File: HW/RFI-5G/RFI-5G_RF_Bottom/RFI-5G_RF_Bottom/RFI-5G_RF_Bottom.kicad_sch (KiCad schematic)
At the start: 20 parts, among them J1 Conn_01x10, J2 Conn_01x10, J3 Conn_01x10, J4 Conn_01x10, J5 SMP, J6 Conn_01x04_Female

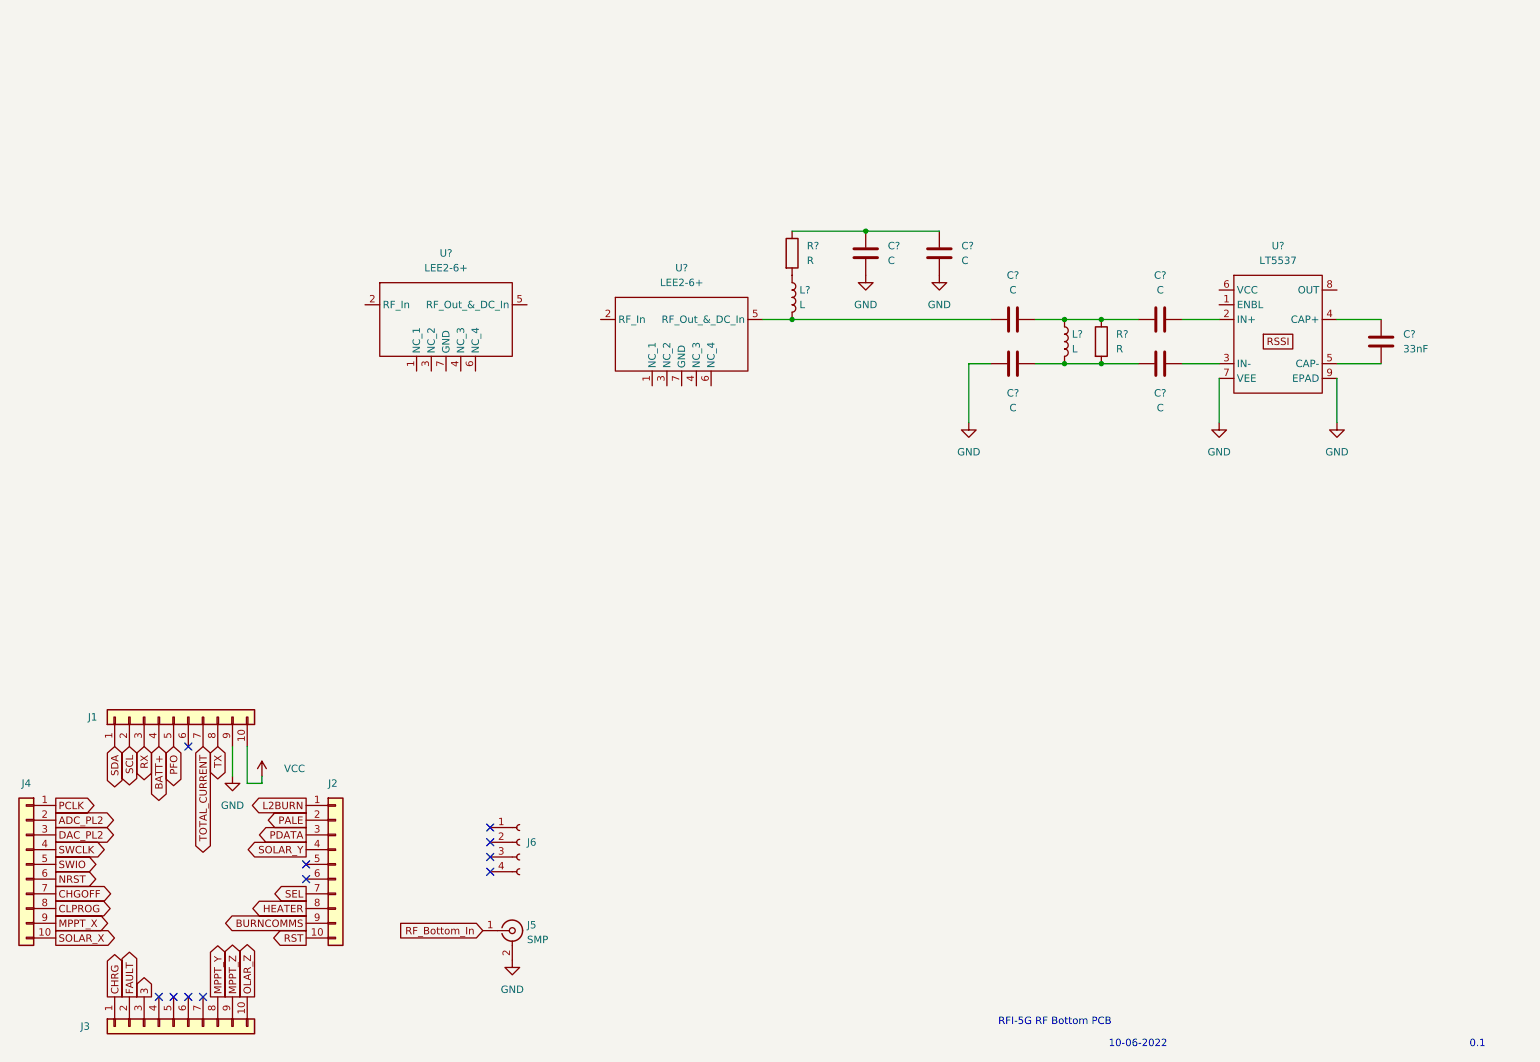
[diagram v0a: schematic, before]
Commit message: RF top and Bottom boards
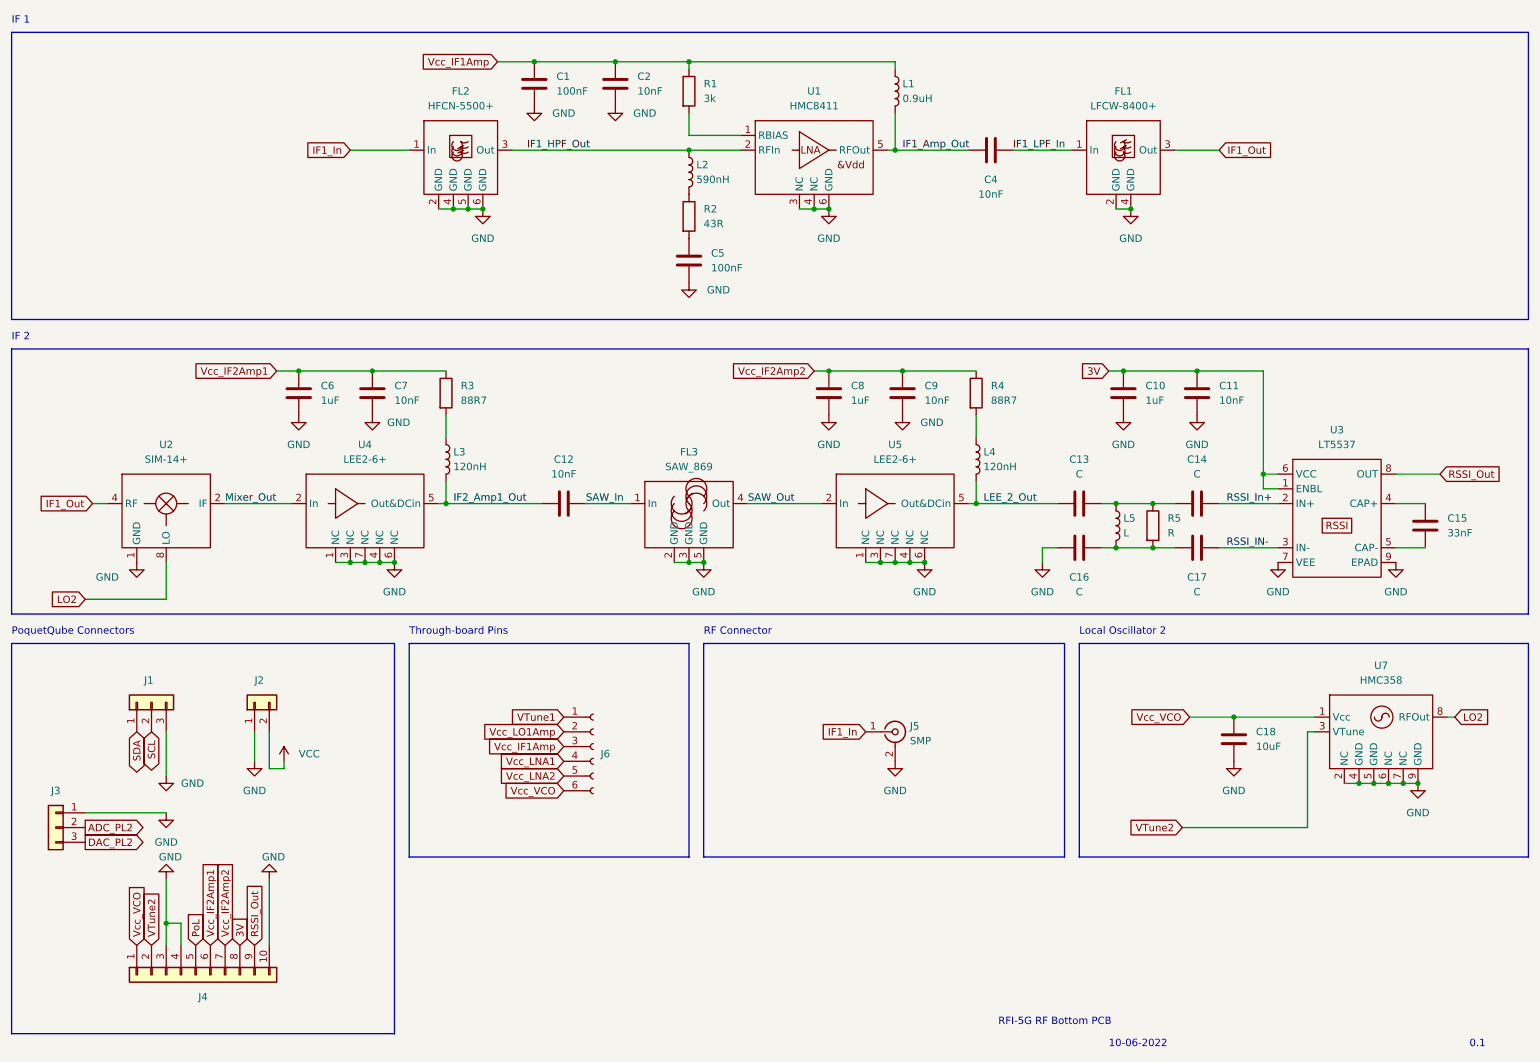
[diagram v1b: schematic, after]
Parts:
- removed J1, J2, J3: Conn_01x10, symbol Connector_Generic:Conn_01x10
- removed J6: Conn_01x04_Female, Connector_PinHeader_2.54mm:PinHeader_1x04_P2.54mm_Vertical, symbol Connector:Conn_01x04_Female
- removed U?: LEE2-6+, Package_SON:WSON-6-1EP_2x2mm_P0.65mm_EP1x1.6mm, symbol GGS_RF:LEE2-6+
- added C1, C5: 100nF, Capacitor_SMD:C_0402_1005Metric, symbol Device:C
- added C10, C6: 1uF, Capacitor_SMD:C_0402_1005Metric, symbol Device:C
- added C11, C12, C2, C4, C7: 10nF, Capacitor_SMD:C_0402_1005Metric, symbol Device:C
- added C18: 10uF, Capacitor_SMD:C_0402_1005Metric, symbol Device:C
- added FL1: LFCW-8400+, GGS_RF:JC0603C-1, symbol GGS_RF:LFCW-8000+
- added FL2: HFCN-5500+, GGS_RF:JC0603C, symbol GGS_RF:HFCN-5500+
- added FL3: SAW_869, GGS_RF:QCS5P, symbol GGS_RF:SAW_869
- added J1, J3: Conn_01x03, Connector_PinHeader_2.54mm:PinHeader_1x03_P2.54mm_Vertical, symbol Connector_Generic:Conn_01x03
- added J2: Conn_01x02, Connector_PinHeader_2.54mm:PinHeader_1x02_P2.54mm_Vertical, symbol Connector_Generic:Conn_01x02
- added J6: Conn_01x06_Female, Connector_PinHeader_1.00mm:PinHeader_1x06_P1.00mm_Vertical, symbol Connector:Conn_01x06_Female
- added L1: 0.9uH, Inductor_SMD:L_0603_1608Metric, symbol Device:L
- added L2: 590nH, Inductor_SMD:L_0603_1608Metric, symbol Device:L
- added L3: 120nH, Inductor_SMD:L_0603_1608Metric, symbol Device:L
- added R1: 3k, Resistor_SMD:R_0603_1608Metric, symbol Device:R
- added R2: 43R, Resistor_SMD:R_0603_1608Metric, symbol Device:R
- added R3: 88R7, Resistor_SMD:R_0603_1608Metric, symbol Device:R
- added U1: HMC8411, GGS_RF:6-LFCSP, symbol GGS_RF:HMC8411
- added U2: SIM-14+, GGS_RF:HV1195, symbol GGS_RF:SIM-14+
- added U4: LEE2-6+, Package_SON:WSON-6-1EP_2x2mm_P0.65mm_EP1x1.6mm, symbol GGS_RF:LEE2-6+
- added U7: HMC358, Package_SO:MSOP-8-1EP_3x3mm_P0.65mm_EP2.5x3mm_Mask1.73x2.36mm, symbol GGS_RF:HMC358
- C8: renamed from C?; value C -> 1uF
- C9: renamed from C?; value C -> 10nF
- J4: footprint (none) -> Connector_PinHeader_2.54mm:PinHeader_1x10_P2.54mm_Vertical
- J5: footprint easyeda:CES-110-XX-Y-S -> GGS_Connectors:SMP_StraightPlugPCB
- L4: renamed from L?; value L -> 120nH; footprint (none) -> Inductor_SMD:L_0603_1608Metric
- L5: renamed from L?; footprint (none) -> Inductor_SMD:L_0603_1608Metric
- R4: renamed from R?; value R -> 88R7; footprint (none) -> Resistor_SMD:R_0603_1608Metric
- R5: renamed from R?; footprint (none) -> Resistor_SMD:R_0603_1608Metric
- gave numbers to parts that had none: 7
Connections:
- net CHGOFF is gone; now on net Vcc_IF2Amp2: J4.7 (Pin_7)
- net CLPROG is gone; now on net 3V: J4.8 (Pin_8)
- net MPPT_X is gone; now on net RSSI_Out: J4.9 (Pin_9)
- net SOLAR_X is gone; now on net GND: J4.10 (Pin_10)
- net SWCLK is gone; now on net GND: J4.4 (Pin_4)
- net ADC_PL2: now also J3.2 (Pin_2); no longer J4.2 (Pin_2)
- net DAC_PL2: now also J3.3 (Pin_3); no longer J4.3 (Pin_3)
- net GND: now also J4.3 (Pin_3), U5.1 (NC), U5.3 (NC), U5.4 (NC), U5.6 (NC), U5.7 (NC), C1.1, C10.1, C11.1, C18.1, C2.1, C5.1, C6.1, C7.1, FL1.2 (GND), FL1.4 (GND), FL2.2 (GND), FL2.4 (GND), FL2.5 (GND), FL2.6 (GND), FL3.2 (GND), FL3.3 (GND), FL3.5 (GND), J1.3 (Pin_3), J2.1 (Pin_1), J3.1 (Pin_1), U1.3 (NC), U1.4 (NC), U1.6 (GND), U2.1 (GND), U4.1 (NC), U4.3 (NC), U4.4 (NC), U4.6 (NC), U4.7 (NC), U7.2 (NC), U7.4 (GND), U7.5 (GND), U7.6 (NC), U7.7 (NC), U7.9 (GND)
- net SCL: now also J1.2 (Pin_2)
- net SDA: now also J1.1 (Pin_1)
- net VCC: now also J2.2 (Pin_2)
- net LEE_2_Out: now reaches C13.1, L4.2, U5.5 (Out&DCin)
- net Vcc_IF2Amp2: now reaches C8.2, C9.2, R4.1
- net 3V: now reaches U3.1 (ENBL)
- net 3V: now also U3.6 (VCC), C10.2, C11.2
- net RSSI_In+: now reaches C14.2, U3.2 (IN+)
- net RSSI_IN-: now reaches C17.2, U3.3 (IN-)
- net RSSI_Out: now reaches U3.8 (OUT)
- net SAW_Out: now reaches U5.2 (In)
- net SAW_Out: now also FL3.4 (Out)
- net NRST renamed Vcc_IF2Amp1
- net Vcc_IF2Amp1: now also C6.2, C7.2, R3.1
- net PCLK renamed Vcc_VCO
- net Vcc_VCO: now also C18.2, J6.6 (Pin_6), U7.1 (Vcc)
- net RF_Bottom_In renamed IF1_In
- net IF1_In: now also FL2.1 (In)
- net SWIO renamed PoL
- new net: L3.1, R3.2
- new net: L2.2, R2.1
- new net: C5.2, R2.2
- new net: R1.2, U1.1 (RBIAS)
- new net IF1_Amp_Out: C4.1, L1.2, U1.5 (RFOut)
- new net IF1_HPF_Out: FL2.3 (Out), L2.1, U1.2 (RFIn)
- new net IF1_LPF_In: C4.2, FL1.1 (In)
- new net IF1_Out: FL1.3 (Out), U2.4 (RF)
- new net IF2_Amp1_Out: C12.1, L3.2, U4.5 (Out&DCin)
- new net LO2: U2.8 (LO), U7.8 (RFOut)
- new net Mixer_Out: U2.2 (IF), U4.2 (In)
- new net SAW_In: C12.2, FL3.1 (In)
- new net VTune1: J6.1 (Pin_1)
- new net VTune2: J4.2 (Pin_2), U7.3 (VTune)
- new net Vcc_IF1Amp: C1.2, C2.2, J6.3 (Pin_3), L1.1, R1.1
- new net Vcc_LNA1: J6.4 (Pin_4)
- new net Vcc_LNA2: J6.5 (Pin_5)
- new net Vcc_LO1Amp: J6.2 (Pin_2)
- no-connect marks 11 -> 0
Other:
- note added: "IF 1"
- note added: "IF 2"
- note added: "Local Oscillator 2"
- note added: "PoquetQube Connectors"
- note added: "RF Connector"
- note added: "Through-board Pins"
- moved on the sheet: C13, C14, C15, C16, C17, C8, C9, J5, L4, L5, R4, R5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
